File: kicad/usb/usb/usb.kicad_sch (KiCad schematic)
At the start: 19 parts, among them J1 USB_C_Receptacle_USB2.0_14P, J2 PH1.25mm 2P, J3 Conn_01x07_Pin, Q1 BSS84, SW1 PWR, U1 S-T111B33MC-OGSTFU, U2 MCP73831-2-OT

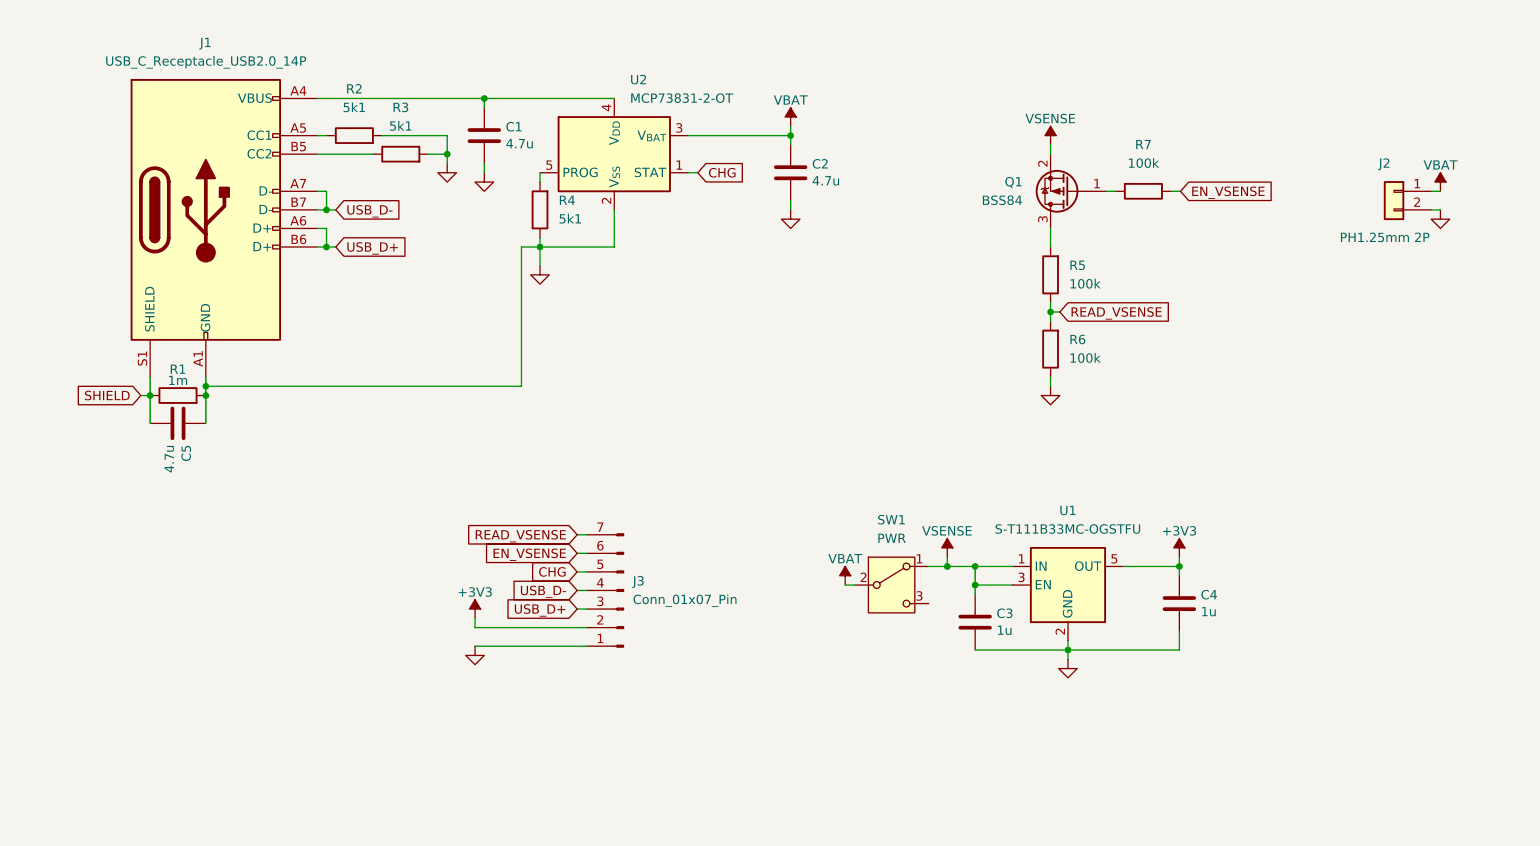
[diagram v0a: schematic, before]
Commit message: Various kicad edits
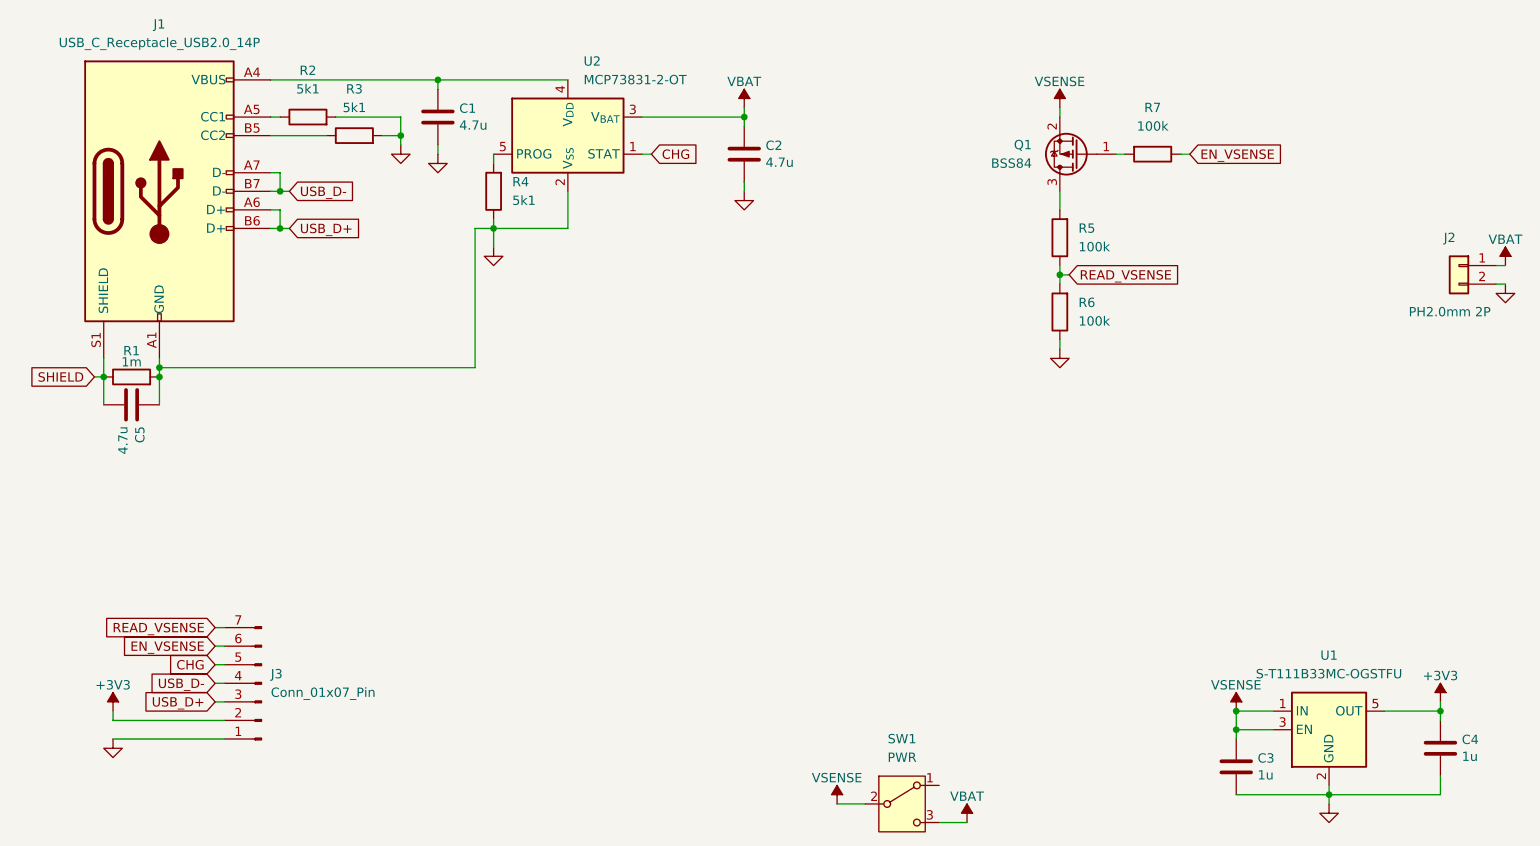
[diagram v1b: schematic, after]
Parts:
- J2: value PH1.25mm 2P -> PH2.0mm 2P; footprint Connector_JST:JST_GH_SM02B-GHS-TB_1x02-1MP_P1.25mm_Horizontal -> Connector_JST:JST_PH_S2B-PH-K_1x02_P2.00mm_Horizontal
- SW1: footprint Button_Switch_SMD:SW_SPDT_Shouhan_MSK12C02 -> Button_Switch_THT:SW_Slide_SPDT_Angled_CK_OS102011MA1Q
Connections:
- net VBAT: now also SW1.3 (C); no longer SW1.2 (B)
- net VSENSE: now also SW1.2 (B); no longer SW1.1 (A)
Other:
- moved on the sheet: C1, C2, C3, C4, C5, J1, J2, J3, Q1, R1, R2, R3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
